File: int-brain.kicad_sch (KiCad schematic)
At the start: 61 parts, among them J1 Right, J10 2MB, J11 1MB, J12 1MA, J13 1MA_ENC, J14 1MB_ENC, J15 2MA_ENC, J16 MPU9250, J17 Conn_01x03, J2 Left, J3 PWR, J4 PWR, J5 USB_A, J6 2MB_ENC, J7 I2C0, J8 UART0, J9 2MA, SW1 SW_Push, U1 PCA9635, U13 AMS1117-3.3, U2 ESP32-DevKitC

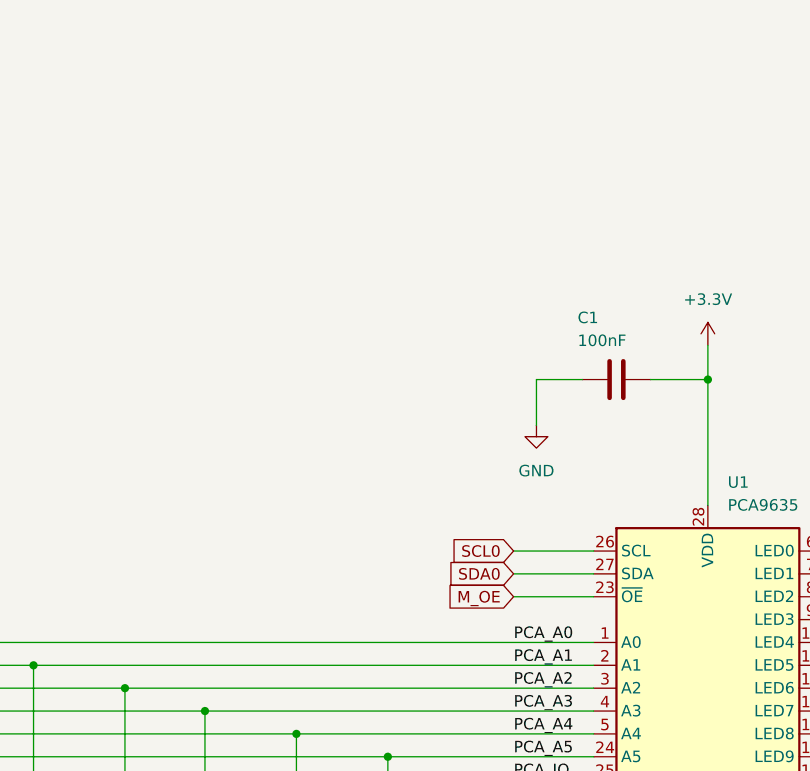
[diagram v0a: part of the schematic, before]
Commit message: done?
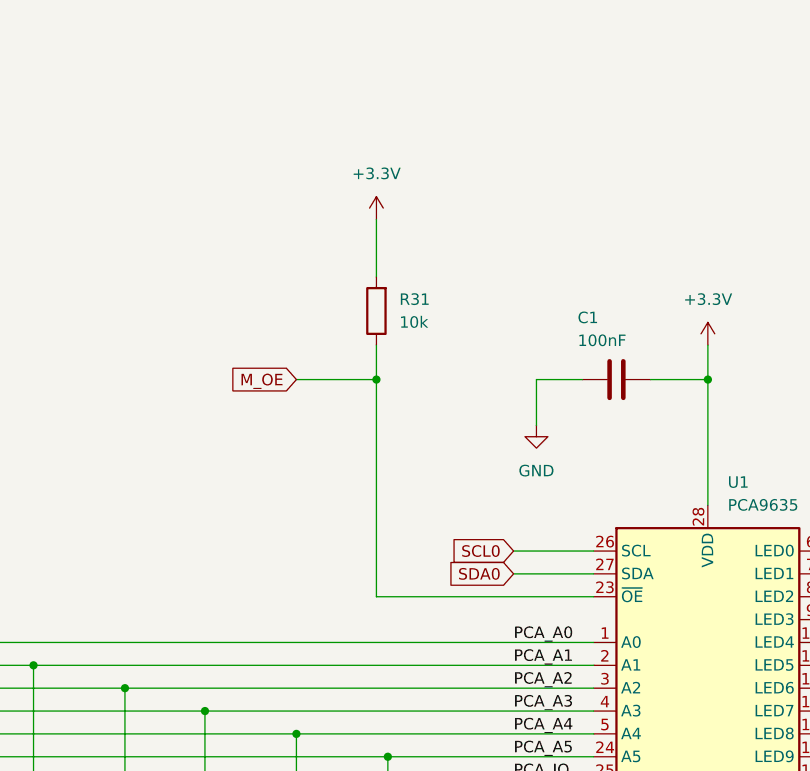
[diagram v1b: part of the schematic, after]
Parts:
- added R31: 10k, Resistor_SMD:R_1206_3216Metric_Pad1.30x1.75mm_HandSolder, symbol Device:R
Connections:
- net +3.3V: now also R31.2
- net M_OE: now also R31.1
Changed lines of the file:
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@@
 	)
 	(junction
+		(at 114.3 354.33)
+		(diameter 0)
+		(color 0 0 0 0)
+	)
+	(junction
 		(at 132.08 463.55)
 		(diameter 0)
@@
 	(wire
 		(pts
+			(xy 114.3 354.33) (xy 114.3 378.46)
+		)
+		(stroke
+			(width 0)
+			(type default)
+		)
+	)
+	(wire
+		(pts
 			(xy 298.45 439.42) (xy 317.5 439.42)
 		)
@@
 	(wire
 		(pts
+			(xy 114.3 336.55) (xy 114.3 342.9)
+		)
+		(stroke
+			(width 0)
+			(type default)
+		)
+	)
+	(wire
+		(pts
 			(xy 50.8 209.55) (xy 97.79 209.55)
 		)
@@
 	(wire
 		(pts
+			(xy 114.3 350.52) (xy 114.3 354.33)
+		)
+		(stroke
+			(width 0)
+			(type default)
+		)
+	)
+	(wire
+		(pts
 			(xy 328.93 163.83) (xy 328.93 158.75)
 		)
@@
 	(wire
 		(pts
-			(xy 129.54 378.46) (xy 138.43 378.46)
+			(xy 105.41 354.33) (xy 114.3 354.33)
 		)
 		(stroke
@@
 	(wire
 		(pts
+			(xy 114.3 378.46) (xy 138.43 378.46)
+		)
+		(stroke
+			(width 0)
+			(type default)
+		)
+	)
+	(wire
+		(pts
 			(xy 322.58 143.51) (xy 322.58 156.21)
 		)
@@
 	(global_label "M_OE"
 		(shape input)
-		(at 129.54 378.46 180)
+		(at 105.41 354.33 180)
 		(fields_autoplaced yes)
 		(effects
@@
 		)
 		(property "Intersheetrefs" "${INTERSHEET_REFS}"
-			(at 121.6563 378.46 0)
+			(at 97.5263 354.33 0)
 			(effects
 				(font
@@
 	)
 	(symbol
+		(lib_id "power:+3.3V")
+		(at 114.3 336.55 0)
+		(unit 1)
+		(exclude_from_sim no)
+		(in_bom yes)
+		(on_board yes)
+		(dnp no)
+		(fields_autoplaced yes)
+		(property "Reference" "#PWR059"
+			(at 114.3 340.36 0)
+			(effects
+				(font
+					(size 1.27 1.27)
+				)
+				(hide yes)
+			)
+		)
+		(property "Value" "+3.3V"
+			(at 114.3 331.47 0)
+			(effects
+				(font
+					(size 1.27 1.27)
+				)
+			)
+		)
+		(property "Footprint" ""
+			(at 114.3 336.55 0)
+			(effects
+				(font
+					(size 1.27 1.27)
+				)
+				(hide yes)
+			)
+		)
+		(property "Datasheet" ""
+			(at 114.3 336.55 0)
+			(effects
+				(font
+					(size 1.27 1.27)
+				)
+				(hide yes)
+			)
+		)
+		(property "Description" "Power symbol creates a global label with name \"+3.3V\""
+			(at 114.3 336.55 0)
+			(effects
+				(font
+					(size 1.27 1.27)
+				)
+				(hide yes)
+			)
+		)
+		(pin "1"
+		)
+		(instances
+			(project "int-brain"
+				(path "/177c6115-ec2a-43b1-88e2-eca3e5dd1279"
+					(reference "#PWR059")
+					(unit 1)
+				)
+			)
+		)
+	)
+	(symbol
 		(lib_id "Jumper:SolderJumper_2_Open")
 		(at 44.45 375.92 0)
@@
 					(unit 1)
 				)
+			)
+		)
+	)
+	(symbol
+		(lib_id "Device:R")
+		(at 114.3 346.71 180)
+		(unit 1)
+		(exclude_from_sim no)
+		(in_bom yes)
+		(on_board yes)
+		(dnp no)
+		(fields_autoplaced yes)
+		(property "Reference" "R31"
+			(at 116.84 345.4399 0)
+			(effects
+				(font
+					(size 1.27 1.27)
+				)
+				(justify right)
+			)
+		)
+		(property "Value" "10k"
+			(at 116.84 347.9799 0)
+			(effects
+				(font
+					(size 1.27 1.27)
+				)
+				(justify right)
+			)
+		)
+		(property "Footprint" "Resistor_SMD:R_1206_3216Metric_Pad1.30x1.75mm_HandSolder"
+			(at 116.078 346.71 90)
+			(effects
+				(font
+					(size 1.27 1.27)
+				)
+				(hide yes)
+			)
+		)
+		(property "Datasheet" "~"
+			(at 114.3 346.71 0)
+			(effects
+				(font
+					(size 1.27 1.27)
+				)
+				(hide yes)
+			)
+		)
+		(property "Description" "Resistor"
+			(at 114.3 346.71 0)
+			(effects
+				(font
+					(size 1.27 1.27)
+				)
+				(hide yes)
+			)
+		)
+		(pin "2"
+		)
+		(pin "1"
+		)
+		(instances
+			(project "int-brain"
+				(path "/177c6115-ec2a-43b1-88e2-eca3e5dd1279"
+					(reference "R31")
+					(unit 1)
+				)

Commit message: minor improvements
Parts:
- D10, D5: value D -> M7
- J1: value Right -> Top
- J17: value Conn_01x03 -> VBATT_SELECT
- J2: value Left -> Bottom
- JP7: value VCC -> I/O
- R30: value 3k9 -> 2k
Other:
- note added: "3.3V LDO"
- note added: "Default I/O to output mode by pull-down."
- note added: "Distriute functionality from the ESP32 to the rest of the board. In general, the signal bus is used to connect headers on either side of the board to access its GPIO and other functionality. Nothing else on the board depends on ESP32 3.3V, so this can be used for peripherals."
- note added: "Drive all motors using PWM signals, sent from the ESP32 using I2C. Eachmotor requires two PWM lines, each corresponding to one pair of the MOSFETs in the H-bridge motor driver. An additional PWM pin has been allocated per motor to indicate speed with LED brightness."
- note added: "ESP32 Microcontroller"
- note added: "I2C address selection is done by pulling down all bits to 0 using a 10k resistor to ground. To make any of them 1, the corresponding solder joint can be filled, and they'll be shorted to 3.3 V."
- note added: "MPU9250 Datasheet: https://invensense.tdk.com/wp-content/uploads/2015/02/ PS-MPU-9250A-01-v1.1.pdf"
- note added: "Motor Logic Section"
- note added: "Note that this +3.3VA is different from the +3.3V used in the rest of the circuit. This is to ensure that the 3.3 V required for the ESP32 is left undisturbed and other components are powered using a dedicated AMS1117-3.3 LDO."
- note added: "PCA9635 datasheet: https://www.nxp.com/docs/en/data-sheet/PCA9635.pdf"
- note added: "Pinout and other information: https://docs.espressif.com/projects/esp-idf/en/stable/esp32/ hw-reference/esp32/get-started-devkitc.html"
- note added: "Power Input Section"
- note added: "Protocol pins (I2C and UART0) are chosen to keep compliance with the Arduino framework, even though this is unlikely to be used with this board. Most other GPIO are chosen based on physical proximity to peripherals and ease of routing the PCB."
- note added: "Provide up to 5V 5A at a USB port, used to drive an SBC such as the Raspberry Pi 5B"
- note added: "SBC Power section"
- note added: "Sensor Module product links - https://robu.in/product/gy-9255-mpu9255-sensor-module/ - https://www.electronicscomp.com/mpu9250-9-axis-gyro- accelerometer-module - https://www.amazon.in/Electrobot-MPU9250-Accelerator- Magnetometer-Arduino/dp/B08R3SXRVH - https://roboticsdna.in/product/gy-87-mpu-9265-3-axis-9-dof- attitude-gyro-magnetometer-accelerator-sensor-module/ - https://rees52.com/products/m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"
- note added: "Support for quadrature rotary encoders is added, in case a compatible motor with encoders can be found. These are connected directly to the ESP32 microcontroller (instead of using another PCA PWM driver) to provide easy configration of hardware interrupts in case this approach is used when programming for the encoders. One JST header for each encoder (one per motor)."
- note added: "Symbol and footprint libraries: https://github.com/espressif/kicad-libraries"
- note added: "Take in 12 V or 24 V (approx; for most calculations, peak values assuming lithium-polymer cells at 4.2 V are considered). Provide basic reverse-polarity protection (diodes) and also reduce to 5V for most of the board's functionality. Provide a voltage reading corresponding to the battery leverl for the microcontroller too."
- note added: "The PCA driver has an active-low enable, so we pull-up to 3.3 V (high) to prevent accidental activation."
- note added: "These ADC pins can only handle input, so they are used for current-sense voltage drops."
- note added: "Use a potential divider to reduce the battery voltage. For various Li-Po batteries, we assume 4.2 V per cell (at full charge). We expect about 3.12 mW - 12.96 mW to be dissipated here. 3S: 47k and 3.9k --> 0.9654223 V 6S: 47k and 2k --> 1.028571429 V The ESP32 seems to read realiably up to around 1 V using the built-in ADCs."
- company: (none) -> Anuj Verma
- title: (none) -> RoboNex
- moved on the sheet: C1, C26, C27, D1, D10, D2, D3, D4, D5, D6, D7, H1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
